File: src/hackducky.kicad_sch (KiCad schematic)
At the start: 46 parts, among them J1 USB_A, J2 Conn_02x02_Top_Bottom, J3 Micro_SD_Card, P2 USB_C_Plug, SW3 BOOT_SEL, SW4 BOOT_SEL, U1 W25Q16JVSS, U2 AP2112K-3.3, U3 USBLC6-2P6, U4 RP2040, U5 USBLC6-2P6, Y1 Crystal_GND24

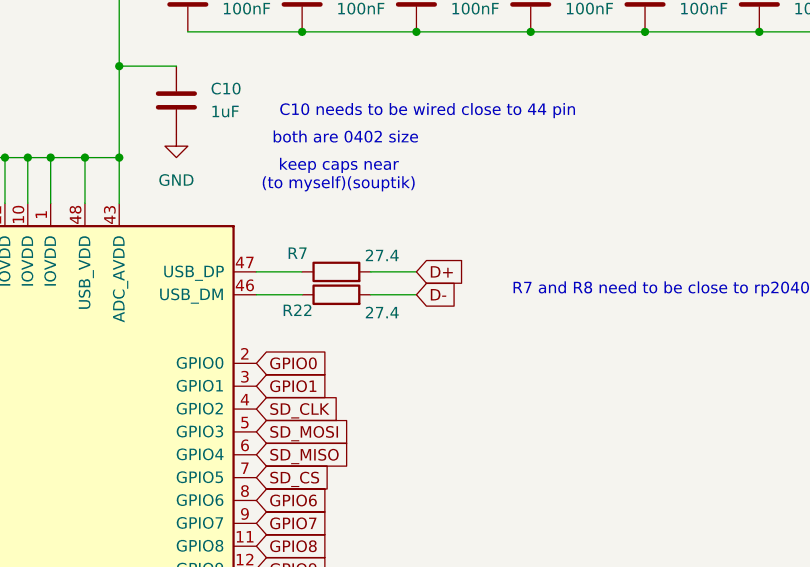
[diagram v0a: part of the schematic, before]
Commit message: update
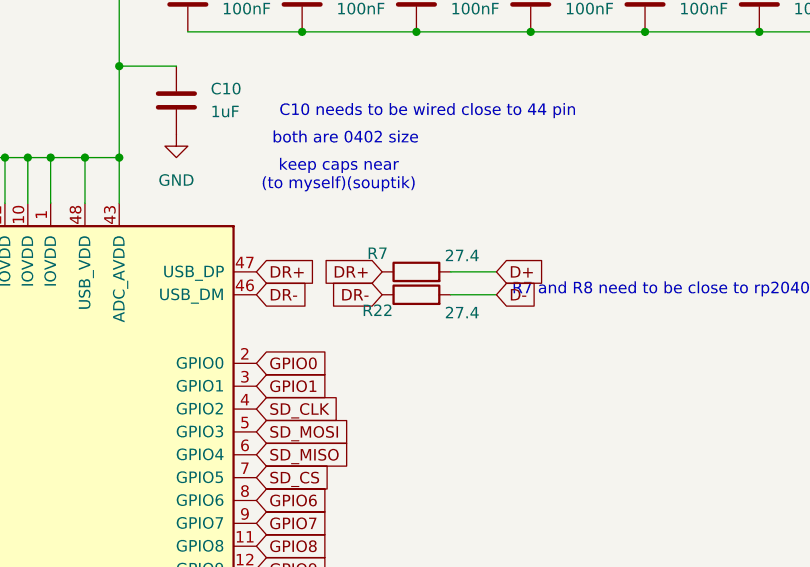
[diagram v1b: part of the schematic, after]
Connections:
- net DR+: now reaches R7.1, U4.47 (USB_DP)
- net DR-: now reaches R22.1, U4.46 (USB_DM)
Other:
- moved on the sheet: R22, R7
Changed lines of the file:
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@@
 	(wire
 		(pts
-			(xy 283.21 85.09) (xy 288.29 85.09)
+			(xy 292.1 85.09) (xy 297.18 85.09)
 		)
 		(stroke
@@
 	(wire
 		(pts
-			(xy 270.51 87.63) (xy 275.59 87.63)
-		)
-		(stroke
-			(width 0)
-			(type default)
-		)
-	)
-	(wire
-		(pts
 			(xy 153.67 341.63) (xy 154.94 341.63)
 		)
@@
 	(wire
 		(pts
-			(xy 283.21 87.63) (xy 288.29 87.63)
+			(xy 292.1 87.63) (xy 297.18 87.63)
 		)
 		(stroke
@@
 	(wire
 		(pts
-			(xy 270.51 85.09) (xy 275.59 85.09)
-		)
-		(stroke
-			(width 0)
-			(type default)
-		)
-	)
-	(wire
-		(pts
 			(xy 195.58 50.8) (xy 208.28 50.8)
 		)
@@
 	(global_label "D+"
 		(shape input)
-		(at 288.29 85.09 0)
+		(at 297.18 85.09 0)
 		(fields_autoplaced yes)
 		(effects
@@
 		)
 		(property "Intersheetrefs" "${INTERSHEET_REFS}"
-			(at 294.1176 85.09 0)
+			(at 303.0076 85.09 0)
 			(effects
 				(font
@@
 		)
 	)
+	(global_label "DR-"
+		(shape input)
+		(at 284.48 87.63 180)
+		(fields_autoplaced yes)
+		(effects
+			(font
+				(size 1.27 1.27)
+			)
+			(justify right)
+		)
+		(property "Intersheetrefs" "${INTERSHEET_REFS}"
+			(at 277.3824 87.63 0)
+			(effects
+				(font
+					(size 1.27 1.27)
+				)
+				(justify right)
+				(hide yes)
+			)
+		)
+	)
 	(global_label "QSPI_SD3"
 		(shape input)
@@
 		)
 	)
+	(global_label "DR+"
+		(shape input)
+		(at 270.51 85.09 0)
+		(fields_autoplaced yes)
+		(effects
+			(font
+				(size 1.27 1.27)
+			)
+			(justify left)
+		)
+		(property "Intersheetrefs" "${INTERSHEET_REFS}"
+			(at 277.6076 85.09 0)
+			(effects
+				(font
+					(size 1.27 1.27)
+				)
+				(justify left)
+				(hide yes)
+			)
+		)
+	)
 	(global_label "GPIO21"
 		(shape input)
@@
 		)
 	)
+	(global_label "DR+"
+		(shape input)
+		(at 284.48 85.09 180)
+		(fields_autoplaced yes)
+		(effects
+			(font
+				(size 1.27 1.27)
+			)
+			(justify right)
+		)
+		(property "Intersheetrefs" "${INTERSHEET_REFS}"
+			(at 277.3824 85.09 0)
+			(effects
+				(font
+					(size 1.27 1.27)
+				)
+				(justify right)
+				(hide yes)
+			)
+		)
+	)
+	(global_label "DR-"
+		(shape input)
+		(at 270.51 87.63 0)
+		(fields_autoplaced yes)
+		(effects
+			(font
+				(size 1.27 1.27)
+			)
+			(justify left)
+		)
+		(property "Intersheetrefs" "${INTERSHEET_REFS}"
+			(at 277.6076 87.63 0)
+			(effects
+				(font
+					(size 1.27 1.27)
+				)
+				(justify left)
+				(hide yes)
+			)
+		)
+	)
 	(global_label "SD_CS"
 		(shape input)
@@
 	(global_label "D-"
 		(shape input)
-		(at 288.29 87.63 0)
+		(at 297.18 87.63 0)
 		(fields_autoplaced yes)
 		(effects
@@
 		)
 		(property "Intersheetrefs" "${INTERSHEET_REFS}"
-			(at 294.1176 87.63 0)
+			(at 303.0076 87.63 0)
 			(effects
 				(font
@@
 	(symbol
 		(lib_id "Device:R")
-		(at 279.4 85.09 90)
+		(at 288.29 85.09 90)
 		(unit 1)
 		(exclude_from_sim no)
@@
 		(dnp no)
 		(property "Reference" "R7"
-			(at 275.082 83.058 90)
+			(at 283.972 83.058 90)
 			(effects
 				(font
@@
 		)
 		(property "Value" "27.4"
-			(at 284.48 83.312 90)
+			(at 293.37 83.312 90)
 			(effects
 				(font
@@
 		)
 		(property "Footprint" "Resistor_SMD:R_0402_1005Metric"
-			(at 279.4 86.868 90)
+			(at 288.29 86.868 90)
 			(effects
 				(font
@@
 		)
 		(property "Datasheet" "~"
-			(at 279.4 85.09 0)
+			(at 288.29 85.09 0)
 			(effects
 				(font
@@
 		)
 		(property "Description" "Resistor"
-			(at 279.4 85.09 0)
+			(at 288.29 85.09 0)
 			(effects
 				(font
@@
 	(symbol
 		(lib_id "Device:R")
-		(at 279.4 87.63 90)
+		(at 288.29 87.63 90)
 		(unit 1)
 		(exclude_from_sim no)
@@
 		(dnp no)
 		(property "Reference" "R22"
-			(at 275.082 89.408 90)
+			(at 283.972 89.408 90)
 			(effects
 				(font
@@
 		)
 		(property "Value" "27.4"
-			(at 284.48 89.662 90)
+			(at 293.37 89.662 90)
 			(effects
 				(font
@@
 		)
 		(property "Footprint" "Resistor_SMD:R_0402_1005Metric"
-			(at 279.4 89.408 90)
+			(at 288.29 89.408 90)
 			(effects
 				(font
@@
 		)
 		(property "Datasheet" "~"
-			(at 279.4 87.63 0)
+			(at 288.29 87.63 0)
 			(effects
 				(font
@@
 		)
 		(property "Description" "Resistor"
-			(at 279.4 87.63 0)
+			(at 288.29 87.63 0)
 			(effects
 				(font
